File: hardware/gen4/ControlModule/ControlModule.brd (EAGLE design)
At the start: 46.4 x 66.3 mm, 39 parts, among them IC1 XMEGA16A4A

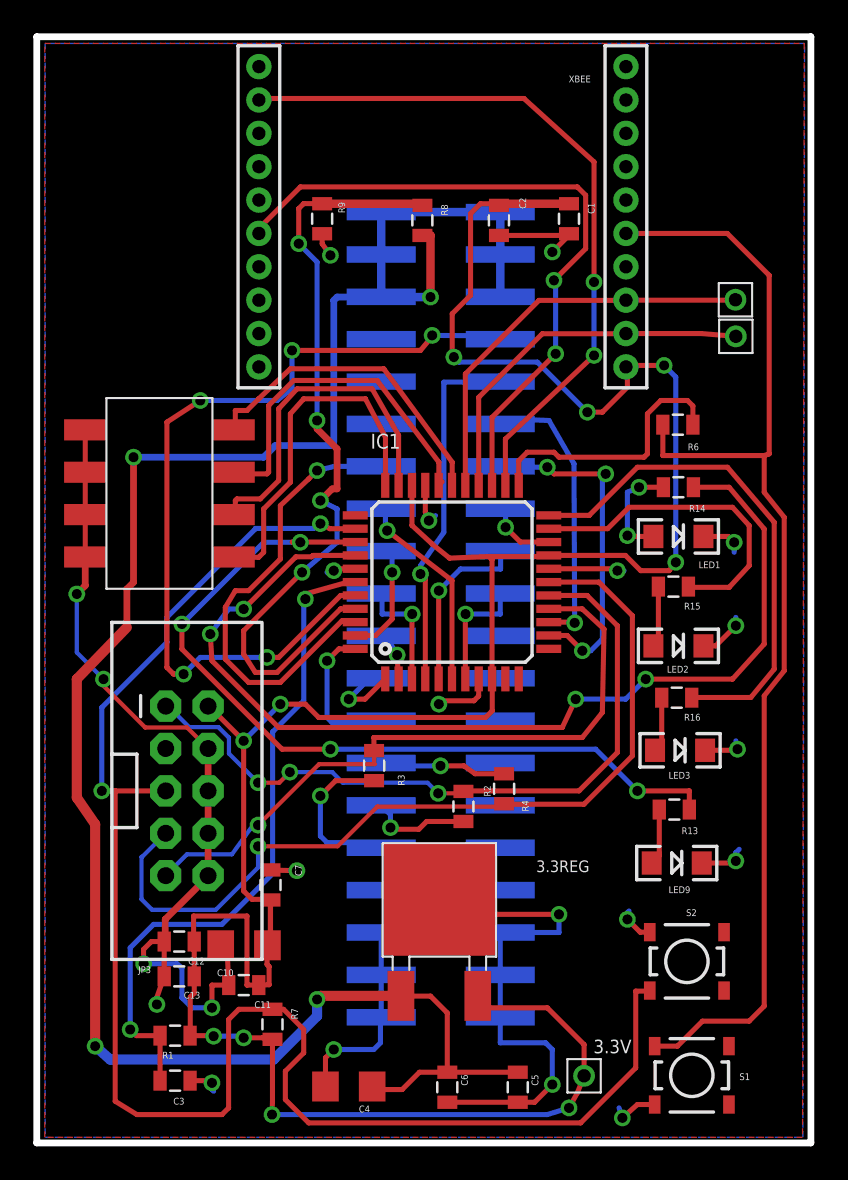
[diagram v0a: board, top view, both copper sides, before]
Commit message: starting routing
done layout
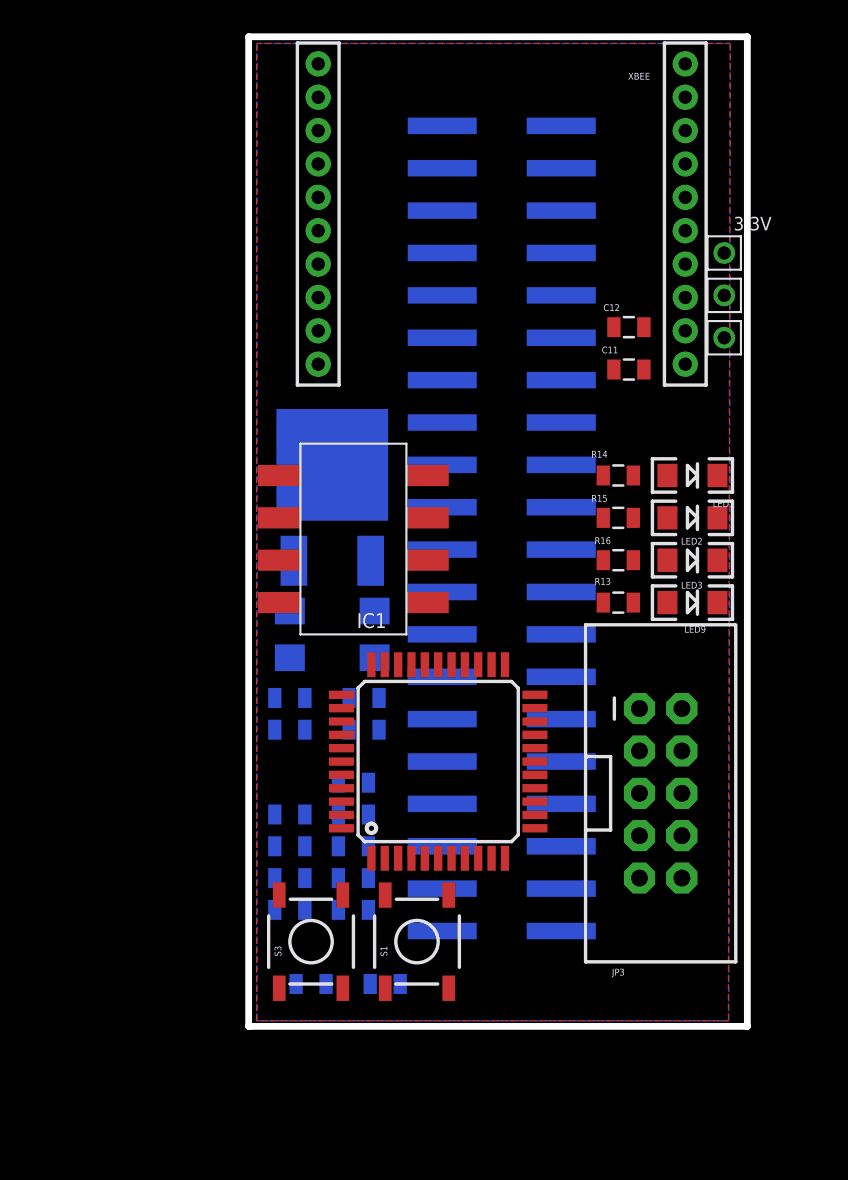
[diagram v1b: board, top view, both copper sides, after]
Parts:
- removed S2: SWITCH-MOMENTARY-2SMD-2, SparkFun-Electromechanical:TACTILE_SWITCH_SMD-2
- added S3: TAC_SWITCHSMD, SparkFun-Retired:TACTILE-SWITCH-SMD
- S1: value SWITCH-MOMENTARY-2SMD-2 -> TAC_SWITCHSMD; device SparkFun-Electromechanical:TACTILE_SWITCH_SMD-2 -> SparkFun-Retired:TACTILE-SWITCH-SMD
- moved 3.3V 50.0 mm to (65.4, 53.3)
- moved C12 45.6 mm to (59.7, 48.9), turned to 180 degrees
- moved C11 43.5 mm to (59.7, 46.4), turned to 180 degrees
- moved R8 41.5 mm to (43.2, 14.0), flipped to the bottom, turned to 0 degrees
- moved C1 41.2 mm to (39.4, 17.8), flipped to the bottom, turned to 0 degrees
- moved R6 40.1 mm to (40.6, 9.53), flipped to the bottom, turned to 0 degrees
- moved R9 39.6 mm to (43.2, 15.9), flipped to the bottom, turned to 180 degrees
- moved C2 37.7 mm to (39.4, 19.7), flipped to the bottom, turned to 180 degrees
- moved JP3 28.4 mm to (61.6, 21.0)
- moved C4 27.3 mm to (39.4, 30.5), flipped to the bottom, turned to 90 degrees
- moved C5 27.0 mm to (39.4, 26.7), flipped to the bottom, turned to 180 degrees
- moved 3.3REG 26.9 mm to (41.9, 40.6), flipped to the bottom
- moved C6 23.4 mm to (39.4, 24.8), flipped to the bottom, turned to 180 degrees
- moved C10 20.2 mm to (44.5, 30.5), flipped to the bottom, turned to 270 degrees
- moved C13 18.5 mm to (43.8, 24.8), flipped to the bottom, turned to 0 degrees
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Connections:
- net GND: now also S1.2, S3.2; no longer S1.1, S2.2
- net RESET: now also S3.4; no longer S2.1
- net XBRST: now also S1.3, S1.4; no longer S1.2
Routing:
- net 3.3V: track 171.0 -> 0.00 mm, vias 10 -> 0
- net 12V: track 122.1 -> 0.00 mm, vias 4 -> 0
- net RESET: track 99.0 -> 0.00 mm, vias 2 -> 0
- net GND: track 94.2 -> 0.00 mm, vias 19 -> 0
- net XBRST: track 70.0 -> 0.00 mm
- net RLED1: track 62.0 -> 0.00 mm, vias 4 -> 0
- net SCK: track 53.1 -> 0.00 mm, vias 1 -> 0
- net BB_IN: track 51.6 -> 0.00 mm, vias 5 -> 0
- net 12VGND: track 50.5 -> 0.00 mm, vias 3 -> 0
- net GLED1: track 49.9 -> 0.00 mm, vias 4 -> 0
- net BATSENSE: track 48.2 -> 0.00 mm, vias 4 -> 0
- net MOSI: track 44.0 -> 0.00 mm, vias 3 -> 0
- net CTS: track 43.3 -> 0.00 mm, vias 2 -> 0
- net RTS: track 40.9 -> 0.00 mm, vias 2 -> 0
- net N$1: track 40.6 -> 0.00 mm, vias 2 -> 0
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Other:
- board size 46.4 x 66.3 mm -> 29.9 x 59.3 mm
